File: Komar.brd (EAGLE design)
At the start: 58 x 58 mm, 109 parts, among them CON1 USB-VERTICAL, CON2 PINHEAD_1X01-2, CON3 CON-4P-TABS-STRAIGHT, CON4 CON-4P-TABS-STRAIGHT, CON5 CON-4P-TABS-STRAIGHT, CON6 CON-4P-TABS-STRAIGHT, CON7 CON-4P-TABS-STRAIGHT, CON8 CON-6P-SM06B, CON9 PINHEAD_1X01-2, IC1 TPD3S014DBVR-SOT23-6, IC2 TPD3S014DBVR-SOT23-6, IC3 ATA6561-GBQW-N-HVSON8, IC4 ATA6561-GBQW-N-HVSON8, IC5 MCP9700AT-E/TTVAO-SOT23, IC6 11LC040T-E/TT, Q1 FDMS86368-F085, Q10 FDMS86368-F085, Q11 FDMS86368-F085, Q12 FDMS86368-F085, Q2 FDMS86368-F085, Q3 FDMS86368-F085, Q4 FDMS86368-F085, Q5 FDMS86368-F085, Q6 FDMS86368-F085, Q7 FDMS86368-F085, Q8 FDMS86368-F085, Q9 FDMS86368-F085

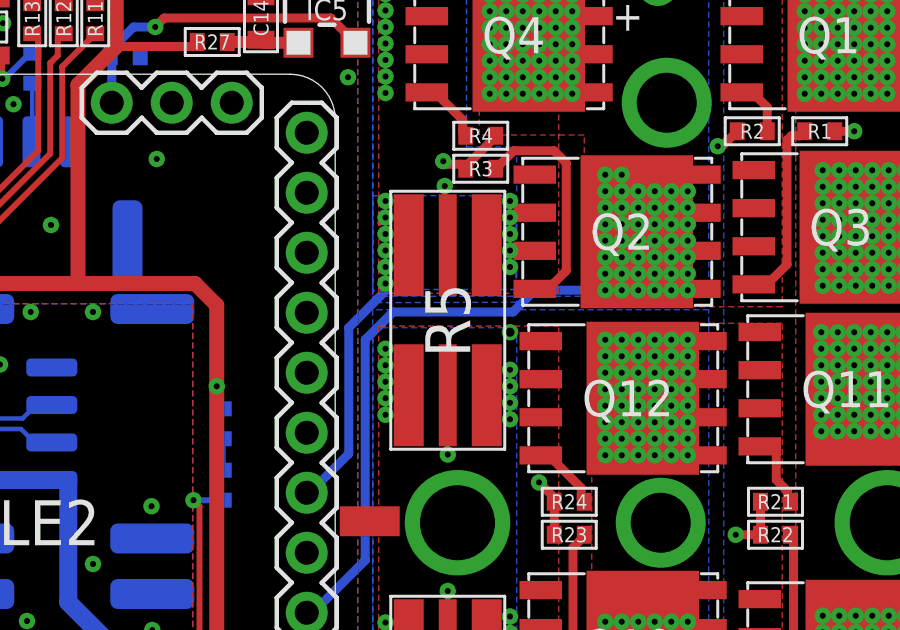
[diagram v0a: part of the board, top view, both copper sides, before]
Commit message: libraries cleanup
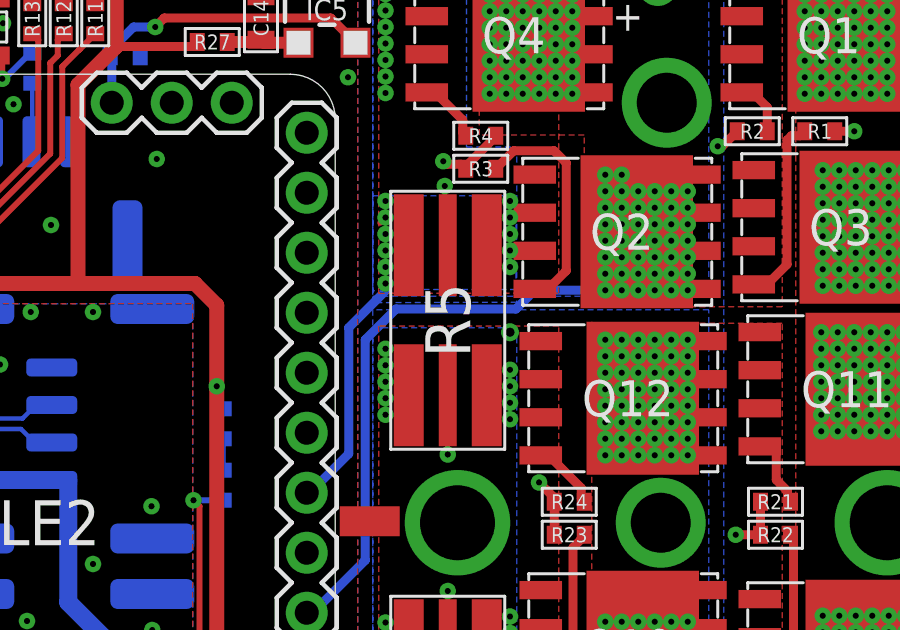
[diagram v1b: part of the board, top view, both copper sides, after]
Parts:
- S1: device macaroni_masterlib:CURRENT_SHUNT_SENSE -> misc:SENSE-0.6
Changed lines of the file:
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@@
 <setting verticaltext="up"/>
 </settings>
-<grid distance="0.05" unitdist="mm" unit="mm" style="lines" multiple="1" display="yes" altdistance="0.1" altunitdist="mm" altunit="mm"/>
+<grid distance="0.1" unitdist="mm" unit="mm" style="lines" multiple="1" display="yes" altdistance="0.1" altunitdist="mm" altunit="mm"/>
 <layers>
 <layer number="1" name="Top" color="4" fill="1" visible="yes" active="yes"/>
-<layer number="2" name="Route2" color="1" fill="3" visible="yes" active="yes"/>
+<layer number="2" name="Route2" color="1" fill="3" visible="no" active="yes"/>
 <layer number="3" name="Route3" color="4" fill="3" visible="no" active="yes"/>
 <layer number="4" name="Route4" color="1" fill="4" visible="no" active="no"/>
@@
 </layers>
 <board>
-<fusionsync huburn="a.cGVyc29uYWw6dWUyYWE4ZDY4" projecturn="a.cGVyc29uYWw6dWUyYWE4ZDY4IzIwMTgxMDI3MTU2OTA4Mjgx" f3durn="urn:adsk.wipprod:dm.lineage:yua-ROE5Tb29pIDQe9ePEg" pcbguid="" lastpulledtime="" lastsyncedchangeguid="2f929fbb-c978-f929-aad6-dc728fd64175" latestrevisionid="943469be-d66c-497d-be2e-a8540f70ffe4" lastsyncedrevisionid="943469be-d66c-497d-be2e-a8540f70ffe4" lastboardhashguid="89bb0dd0-0cd7-6a5e-7a1a-cabf21d338ab" lastpushedtime="2020-05-12T09:11:51Z" linktopcb3d="%12"/>
 <plain>
 <wire x1="29.2" y1="56.85" x2="29.2" y2="1.15" width="0.2" layer="22" style="shortdash"/>
@@
 <attribute name="TOLERANCE" value="5%" x="-160.25" y="-11.3" size="1.778" layer="27" display="off"/>
 </element>
-<element name="S1" library="macaroni_masterlib" package="CURRENT_SHUNT_SENSE" value="SENSE" x="34.775" y="35.35" smashed="yes">
+<element name="S1" library="misc" library_urn="urn:adsk.eagle:library:5347860" package="SENSE-0.6" package3d_urn="urn:adsk.eagle:package:7365871/1" value="SENSE" x="34.775" y="35.35" smashed="yes">
 <attribute name="BOM" value="EXCLUDE" x="-183.225" y="-31.65" size="1.778" layer="27" display="off"/>
 </element>
@@
 <wire x1="28" y1="26" x2="28.2" y2="26" width="0.3" layer="16"/>
 <wire x1="35.6" y1="36.75" x2="37.95" y2="36.75" width="0.3" layer="16"/>
-<wire x1="29.95" y1="35.1" x2="30.875" y2="36.025" width="0.3" layer="16"/>
-<wire x1="30.875" y1="36.025" x2="34.875" y2="36.025" width="0.3" layer="16"/>
-<wire x1="34.875" y1="36.025" x2="35.6" y2="36.75" width="0.3" layer="16"/>
+<wire x1="29.95" y1="35.1" x2="30.975" y2="36.125" width="0.3" layer="16"/>
+<wire x1="30.975" y1="36.125" x2="34.975" y2="36.125" width="0.3" layer="16"/>
+<wire x1="34.975" y1="36.125" x2="35.6" y2="36.75" width="0.3" layer="16"/>
 <wire x1="28.2" y1="26" x2="29.95" y2="27.75" width="0.3" layer="16"/>
 <wire x1="29.95" y1="27.75" x2="29.95" y2="35.1" width="0.3" layer="16"/>
@@
 </note>
 <note version="8.3" severity="warning">
-Since Version 8.3, EAGLE supports Fusion synchronisation.
-This feature will not be available in this version and saving
-the document will break the link to the Fusion PCB feature.
-</note>
-<note version="8.3" severity="warning">
